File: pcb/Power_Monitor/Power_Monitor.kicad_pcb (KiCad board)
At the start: 2 copper layers, 33.6 x 32.4 mm, 14 parts, among them J1 XT60, J2 JST1.25, U1 INA226

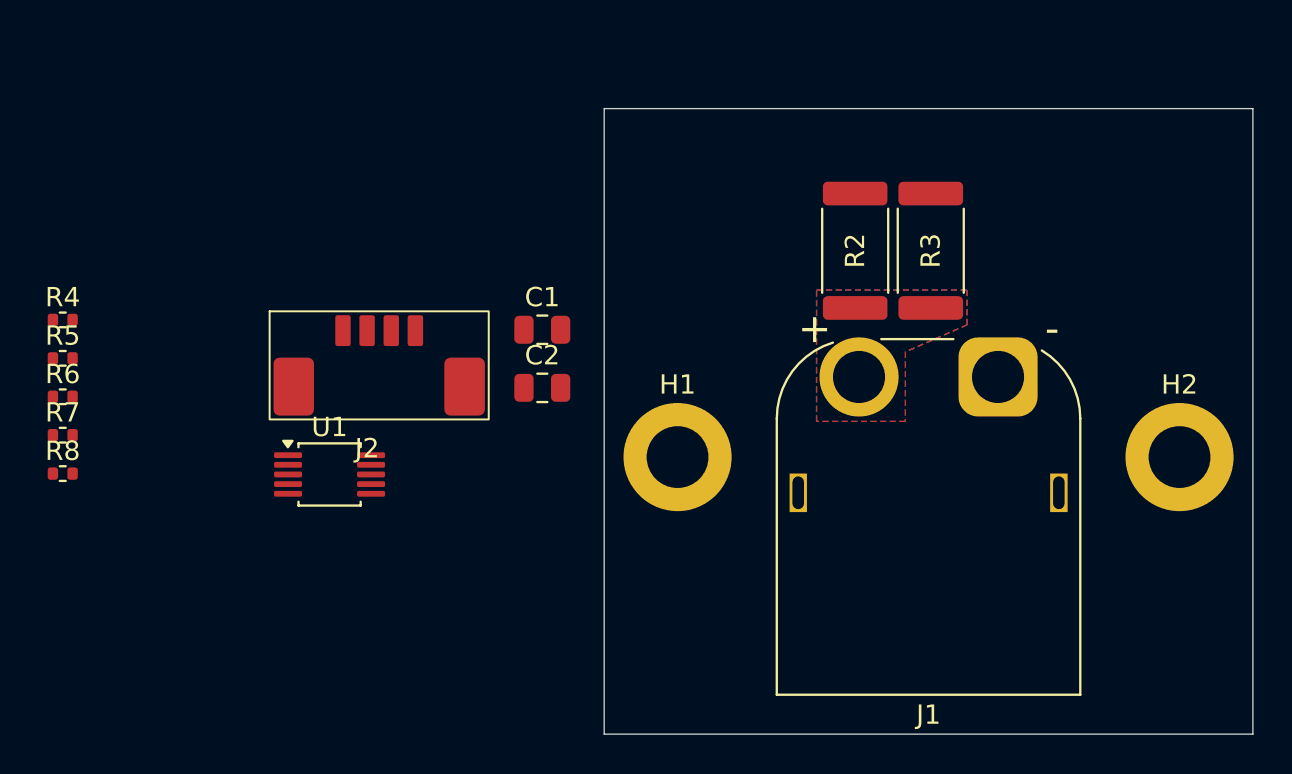
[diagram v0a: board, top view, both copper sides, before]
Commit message: rtos architecture
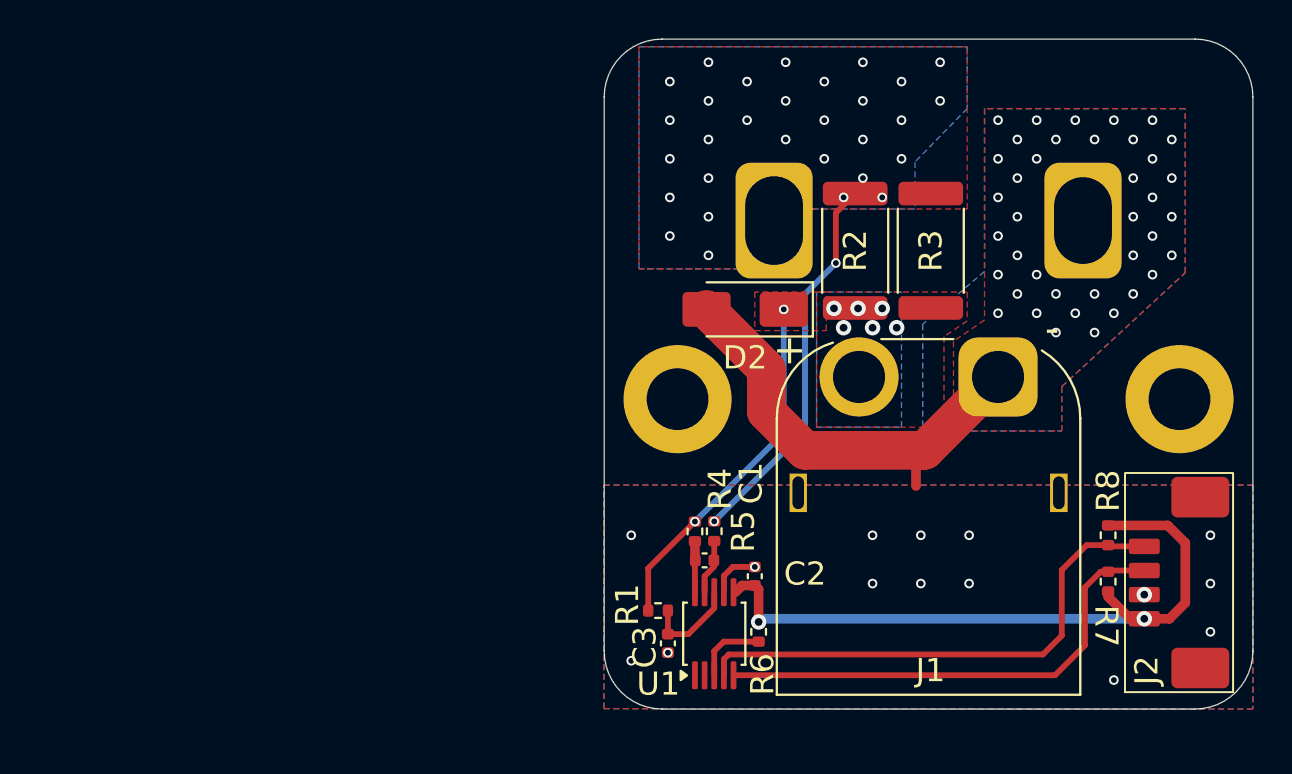
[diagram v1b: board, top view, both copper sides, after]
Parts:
- added C3: 0.1u, Capacitor_SMD:C_0402_1005Metric, F.Cu at (111.9, 123.1)
- added D2: SMAJ15A, Diode_SMD:D_SMA, F.Cu at (115.9, 105.8)
- added G***: LOGO, Local Footprints:logo1, B.Cu at (133.8, 121.3)
- added J3: Castellated Pad, Local Footprints:Castellated_pad_high_side, F.Cu at (117.4, 101.2)
- added J4: Castellated Pad, Local Footprints:Castellated_pad_low_side, F.Cu at (133.4, 101.2)
- added NT1: NetTie_2, NetTie:NetTie-2_SMD_Pad0.5mm, F.Cu at (124.8, 114.5)
- added R1: 10R, Resistor_SMD:R_0402_1005Metric, F.Cu at (111.4, 121.4)
- C1, C2: footprint Capacitor_SMD:C_0805_2012Metric -> Capacitor_SMD:C_0402_1005Metric
- moved R7 54.7 mm to (134.7, 119.9), turned to -90 degrees
- moved R8 54.2 mm to (134.7, 117.5), turned to 90 degrees
- moved J2 44.1 mm to (136.6, 121.8), turned to 90 degrees
- moved R6 38.0 mm to (116.6, 122.5), turned to 90 degrees
- moved R5 34.9 mm to (114.3, 117.3), turned to -90 degrees
- moved R4 34.5 mm to (113.3, 117.3), turned to -90 degrees
- moved U1 21.6 mm to (114.3, 122.6), turned to 90 degrees
- moved C2 14.7 mm to (116.4, 119.6), turned to 90 degrees
- moved C1 14.6 mm to (113.8, 118.8)
- moved H1 3.00 mm to (112.4, 110.5)
- moved H2 3.00 mm to (138.4, 110.5)
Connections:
- C2 pad 2: GND -> GND2
- J1 pad 1: GND -> GND1
- J1 pad 2: Net-(J1-Pin_2) -> Net-(D2-A1)
- J2 pad 2: GND -> GND2
- R2 pad 1: Net-(J1-Pin_2) -> Net-(D2-A1)
- R3 pad 1: Net-(J1-Pin_2) -> Net-(D2-A1)
- R4 pad 1: Net-(J1-Pin_2) -> Net-(D2-A1)
- U1 pad 7: GND -> GND2
- U1 pad 8: Net-(J1-Pin_2) -> Net-(U1-Vbus)
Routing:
- net +3V3: track 0.00 -> 35.7 mm, vias 0 -> 2
- net /SDA: track 0.00 -> 27.1 mm
- net /SCL: track 0.00 -> 25.3 mm
- net GND1: track 0.00 -> 21.0 mm, vias 0 -> 39
- net Net-(J3-Pin_1): track 0.00 -> 20.0 mm, vias 0 -> 32
- net Net-(D2-A1): track 0.00 -> 18.5 mm, vias 0 -> 8
- net Net-(U1-Vbus): track 0.00 -> 5.00 mm
- net Net-(U1-~{Alert}): track 0.00 -> 3.75 mm
- net Net-(U1-Vin-): track 0.00 -> 2.86 mm
- net Net-(U1-Vin+): track 0.00 -> 2.66 mm
- net GND2: track 0.00 -> 2.64 mm, vias 0 -> 15
- added copper zone on B.Cu, net GND1
- added copper zone on F.Cu, net GND1
- added copper zone on B.Cu, net GND2
- added copper zone on F.Cu, net GND2
- added copper zone on B.Cu, net Net-(D2-A1)
- added copper zone on F.Cu, net Net-(D2-A1)
- added copper zone on B.Cu, net Net-(J3-Pin_1)
- added copper zone on F.Cu, net Net-(J3-Pin_1)
- removed copper zone on B.Cu, net Net-(J1-Pin_2)
- removed copper zone on F.Cu, net Net-(J1-Pin_2)
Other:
- board size 33.6 x 32.4 mm -> 33.6 x 34.7 mm
- board text added: "Metrology Lab"
- board text added: "OISP Drone"
